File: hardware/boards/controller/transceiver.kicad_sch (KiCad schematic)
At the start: 30 parts, among them J6 SMA, U7 NRF24L01, U8 RFX2401C, Y3 16MHz

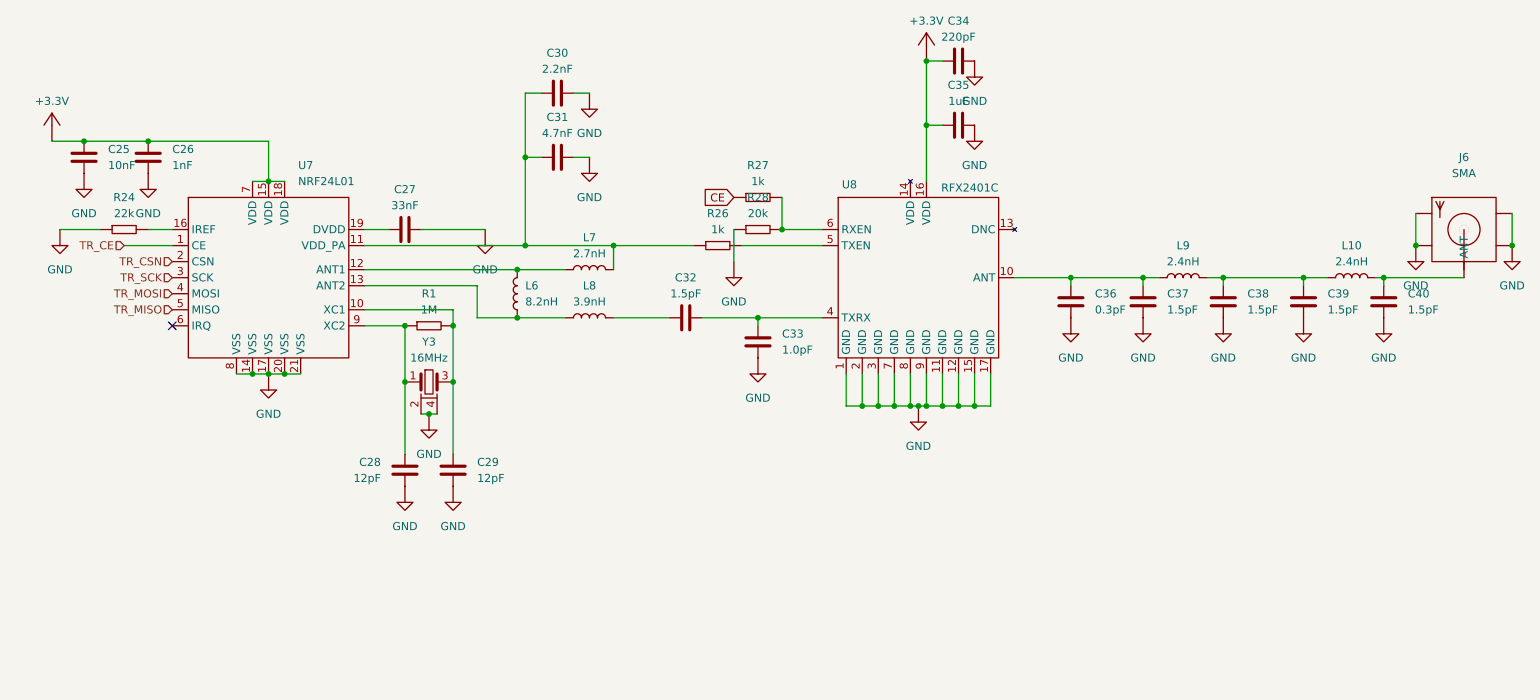
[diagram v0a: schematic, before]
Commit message: new version for pcb controller
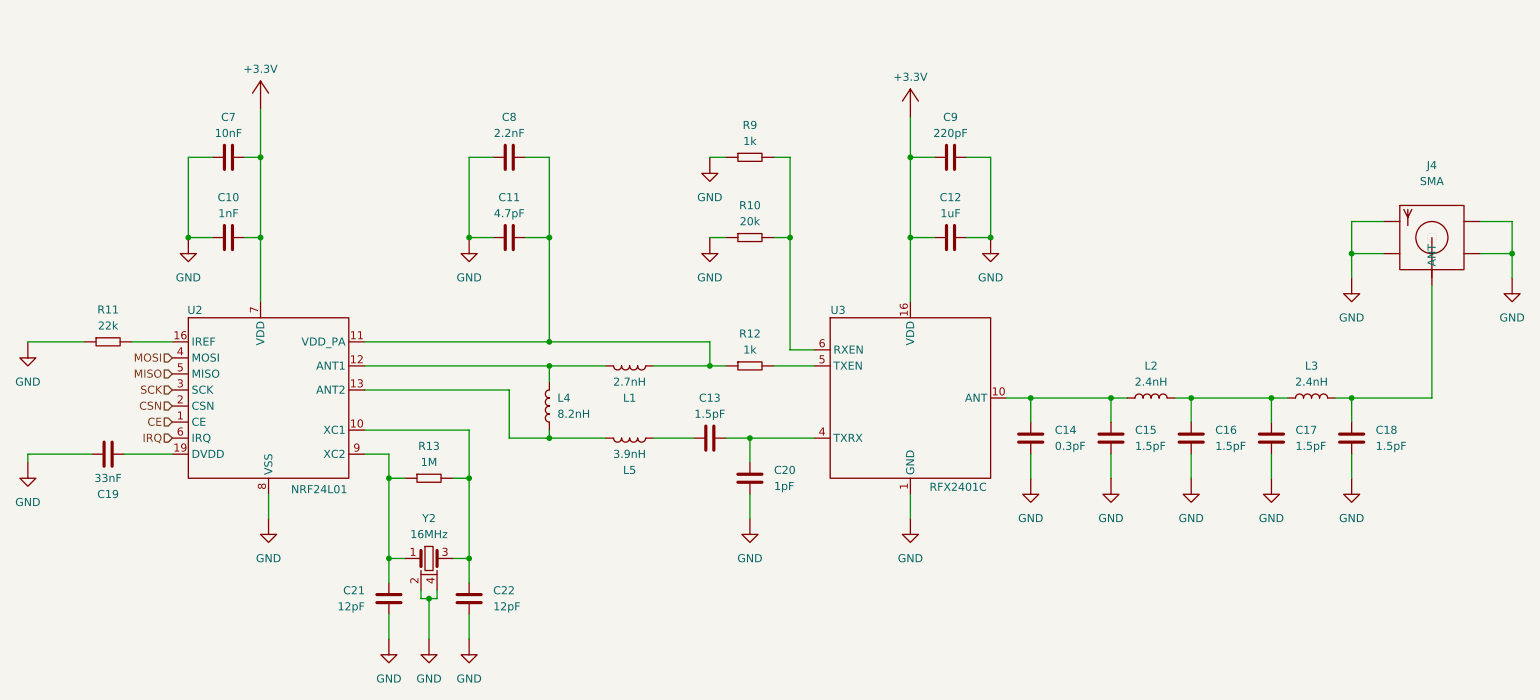
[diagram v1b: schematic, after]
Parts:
- removed L7: 2.7nH, common:L_0603, symbol common:Inductor
- removed L8: 3.9nH, common:L_0603, symbol common:Inductor
- added L1: 2.7nH, common:L_0603, symbol common:Inductor
- added L5: 3.9nH, common:L_0603, symbol common:Inductor
- C11: renamed from C31; value 4.7nF -> 4.7pF
- C20: renamed from C33; value 1.0pF -> 1pF
- renumbered C26 to C10, C35 to C12, C32 to C13, C36 to C14, C37 to C15, C38 to C16, C39 to C17, C40 to C18, C27 to C19, C28 to C21, C29 to C22, C25 to C7, C30 to C8, C34 to C9, J6 to J4, L9 to L2, L10 to L3, L6 to L4, R28 to R10, R24 to R11, R26 to R12, R1 to R13, R27 to R9, U7 to U2, U8 to U3, Y3 to Y2
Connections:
- net TR_CE is gone; now on net CE: U2.1 (CE)
- net +3.3V: now also C10.1, C7.1; no longer C10.2, C7.2
- net CE: no longer R9.1
- net GND: now also C10.2, C11.1, C19.1, C7.2, C8.1, R9.1; no longer C10.1, C11.2, C19.2, C7.1, C8.2
- net at R12.1, U2.11 (VDD_PA): now also C11.2, C8.2, L1.1; no longer C11.1, C8.1
- net at L4.2, U2.12 (ANT1): now also L1.2
- net at L4.1, U2.13 (ANT2): now also L5.2
- net at U2.19 (DVDD): now also C19.2; no longer C19.1
- net IRQ: now reaches U2.6 (IRQ)
- net at C13.1: now also L5.1
- net TR_CSN renamed CSN
- net TR_MISO renamed MISO
- net TR_MOSI renamed MOSI
- net TR_SCK renamed SCK
- no-connect marks 1 -> 0
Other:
- moved on the sheet: C10, C11, C12, C13, C14, C15, C16, C17, C18, C19, C20, C21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
